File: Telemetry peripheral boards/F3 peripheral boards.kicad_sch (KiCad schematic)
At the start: 39 parts, among them J1 ATS668LSM, J2 Conn_01x04_MountingPin, J3 Potentiometer, J4 Strain Gauge, U1 LM2907M/NOPB, U2 INA125U, U3 MCP2515-I/SO, U4 ISO1050DUB, U5 ATTINY1616-MNR, U6 LM7805_TO220, U7 LD1117V33C

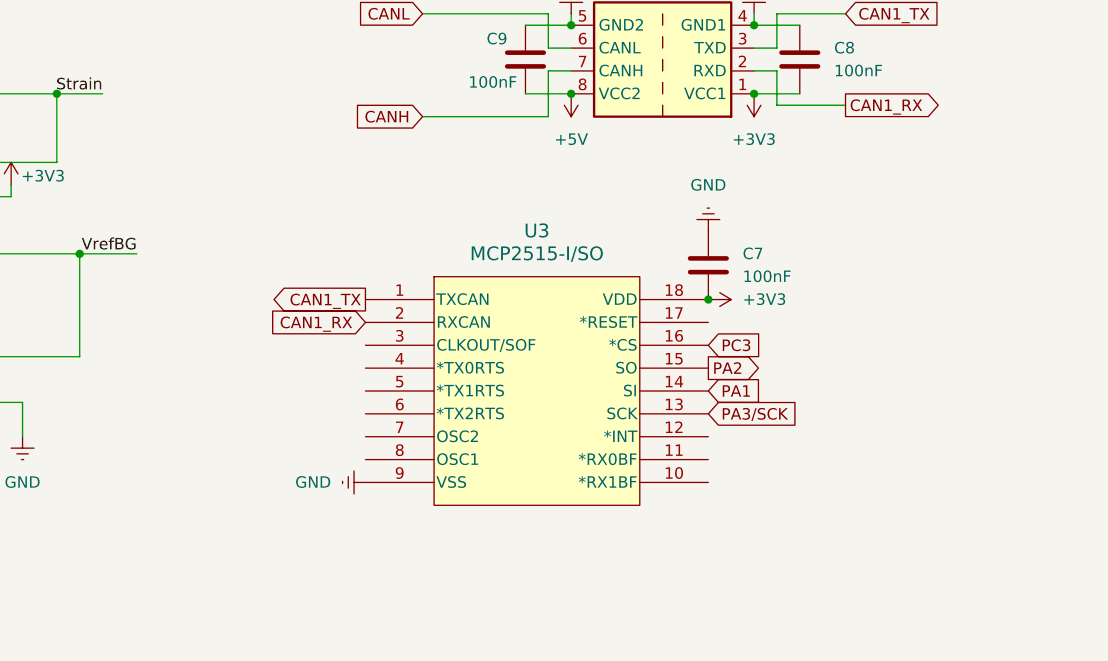
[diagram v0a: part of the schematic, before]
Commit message: updated can controller
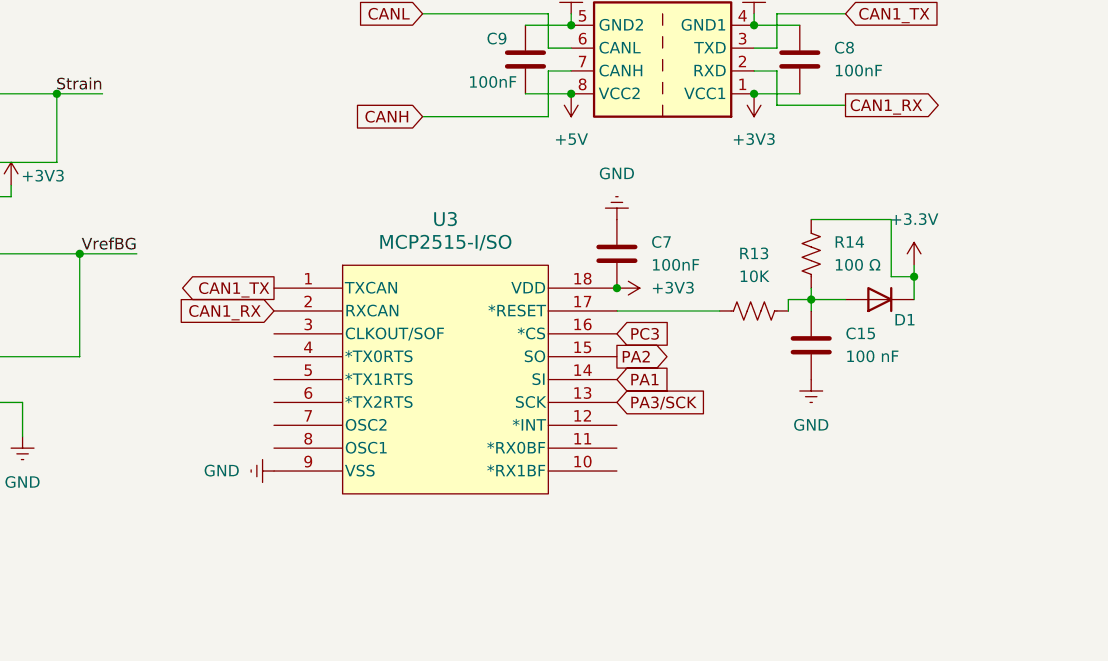
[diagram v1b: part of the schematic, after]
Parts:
- added C15: 100 nF, Capacitor_SMD:C_0805_2012Metric_Pad1.18x1.45mm_HandSolder, symbol Device:C
- added D1: D, Diode_SMD:D_0805_2012Metric, symbol Device:D
- added R13: 10K, Resistor_SMD:R_0805_2012Metric_Pad1.20x1.40mm_HandSolder, symbol Device:R_US
- added R14: 100 Ω, Resistor_SMD:R_0805_2012Metric_Pad1.20x1.40mm_HandSolder, symbol Device:R_US
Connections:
- net GND: now also C15.2
- net at U3.17 (*RESET): now also R13.1
- new net: C15.1, D1.2 (A), R13.2, R14.2
- new net +3.3V: D1.1 (K), R14.1
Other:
- moved on the sheet: C7, U3

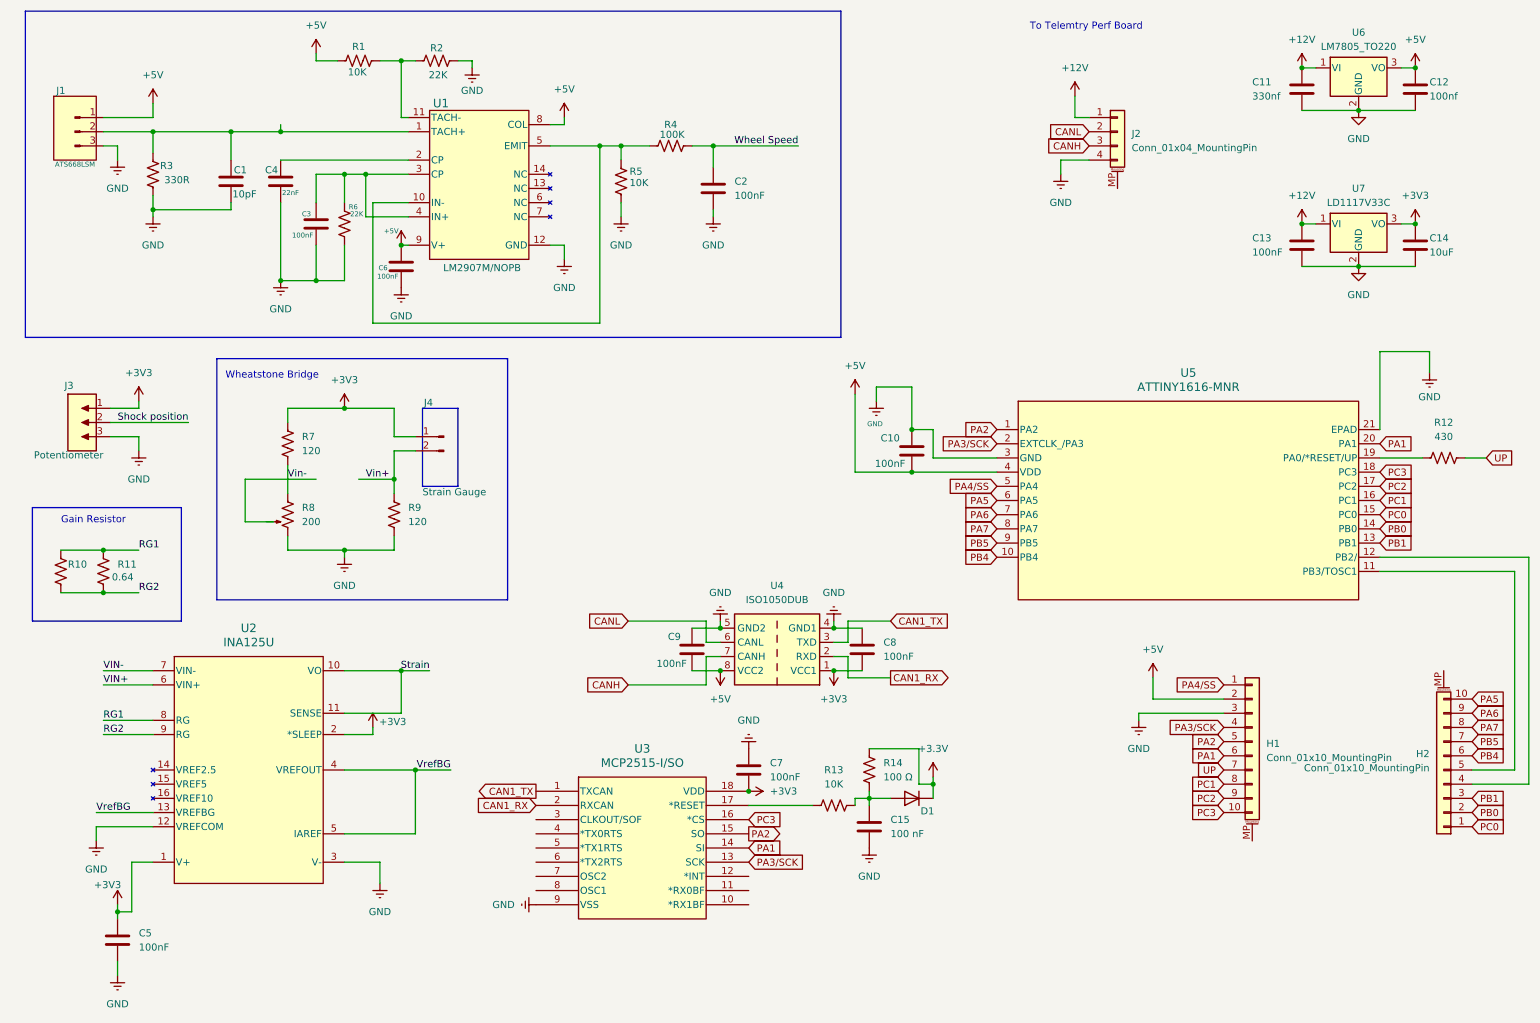
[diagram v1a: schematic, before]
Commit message: PCB for peripheral boards
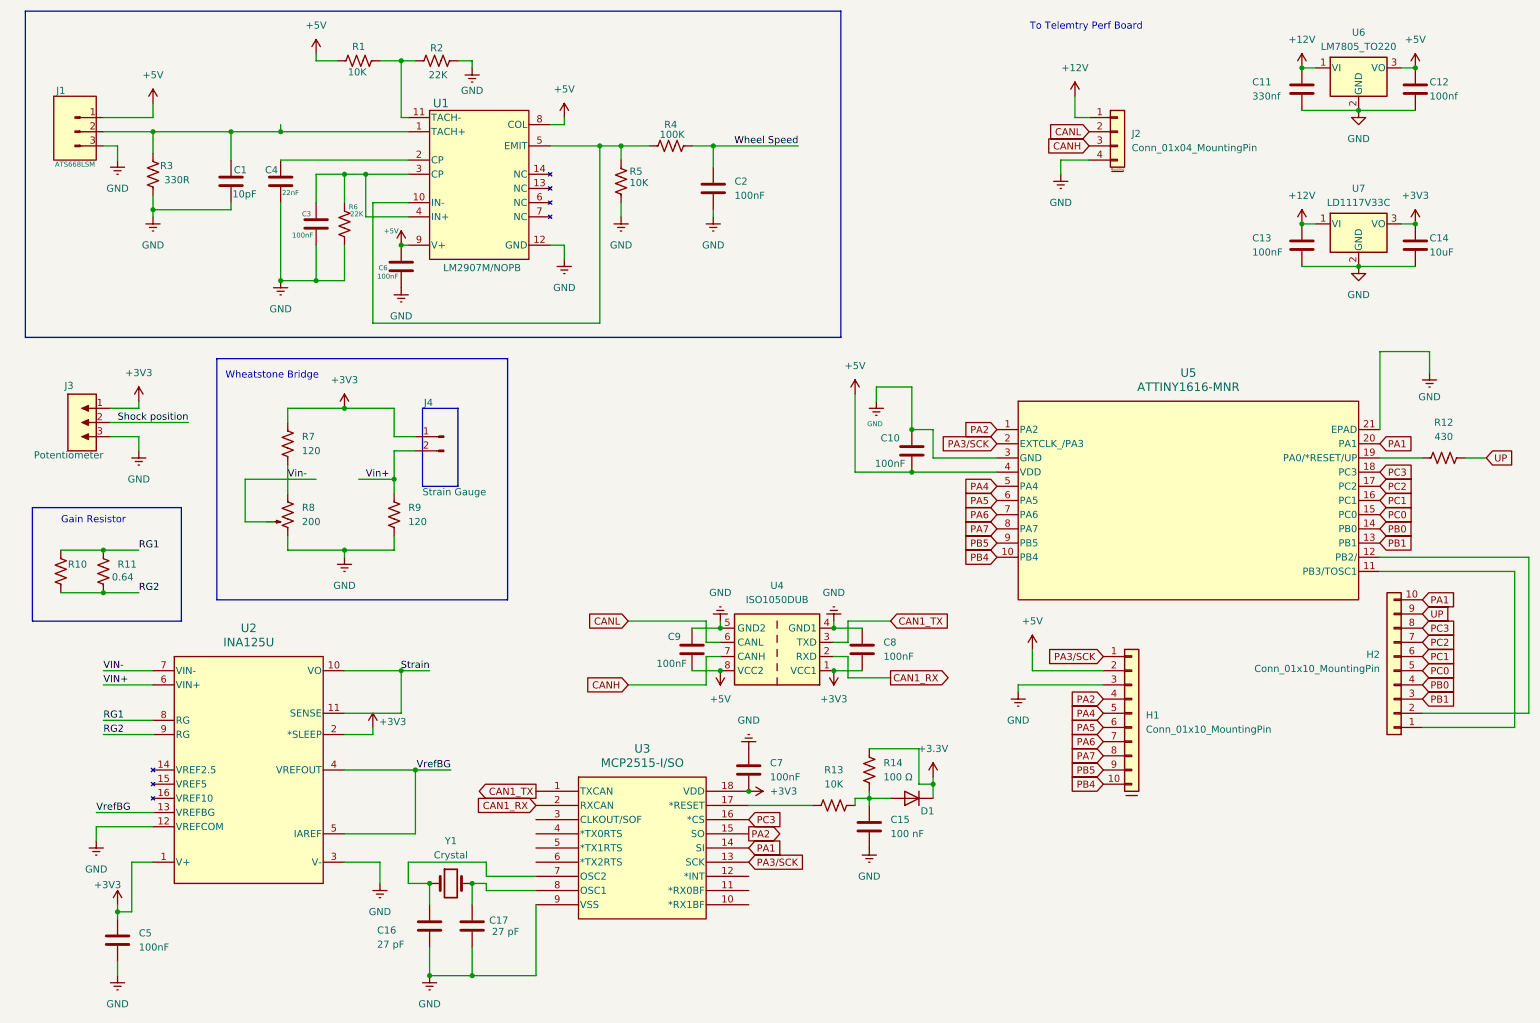
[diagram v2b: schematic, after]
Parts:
- added C16, C17: 27 pF, Capacitor_SMD:C_0805_2012Metric_Pad1.18x1.45mm_HandSolder, symbol Device:C
- added Y1: Crystal, Crystal:Crystal_SMD_5032-2Pin_5.0x3.2mm_HandSoldering, symbol Device:Crystal
- H1: footprint (none) -> Connector_PinHeader_1.00mm:PinHeader_1x10_P1.00mm_Vertical
- J1: footprint (none) -> Connector_PinHeader_2.00mm:PinHeader_1x03_P2.00mm_Vertical
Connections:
- net GND: now also C16.2, C17.2
- net PA1: now also H2.10 (Pin_10); no longer H1.6 (Pin_6)
- net PA2: now also H1.4 (Pin_4); no longer H1.5 (Pin_5)
- net PA3/SCK: now also H1.1 (Pin_1); no longer H1.4 (Pin_4)
- net PA5: now also H1.6 (Pin_6); no longer H2.10 (Pin_10)
- net PA6: now also H1.7 (Pin_7); no longer H2.9 (Pin_9)
- net PA7: now also H1.8 (Pin_8); no longer H2.8 (Pin_8)
- net PB0: now also H2.4 (Pin_4); no longer H2.2 (Pin_2)
- net PB4: now also H1.10 (Pin_10); no longer H2.6 (Pin_6)
- net PB5: now also H1.9 (Pin_9); no longer H2.7 (Pin_7)
- net PC0: now also H2.5 (Pin_5); no longer H2.1 (Pin_1)
- net PC1: now also H2.6 (Pin_6); no longer H1.8 (Pin_8)
- net PC2: now also H2.7 (Pin_7); no longer H1.9 (Pin_9)
- net PC3: now also H2.8 (Pin_8); no longer H1.10 (Pin_10)
- net UP: now also H2.9 (Pin_9); no longer H1.7 (Pin_7)
- net at U5.11 (PB3/TOSC1): now also H2.1 (Pin_1); no longer H2.5 (Pin_5)
- net at U5.12 (PB2/): now also H2.2 (Pin_2); no longer H2.4 (Pin_4)
- net at U3.7 (OSC2): now also C16.1, Y1.1
- net at U3.8 (OSC1): now also C17.1, Y1.2
- net PA4/SS renamed PA4
- net PA4: now also H1.5 (Pin_5); no longer H1.1 (Pin_1)

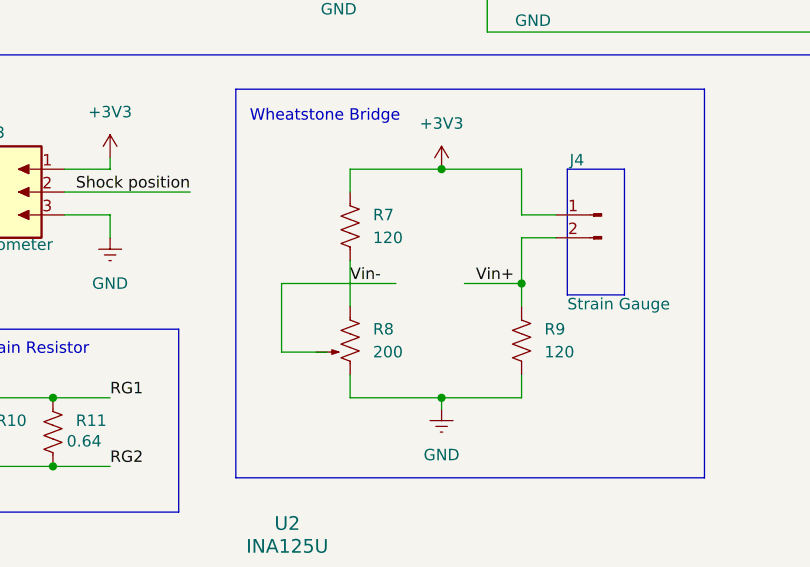
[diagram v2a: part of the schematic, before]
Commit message: Peripheral boards
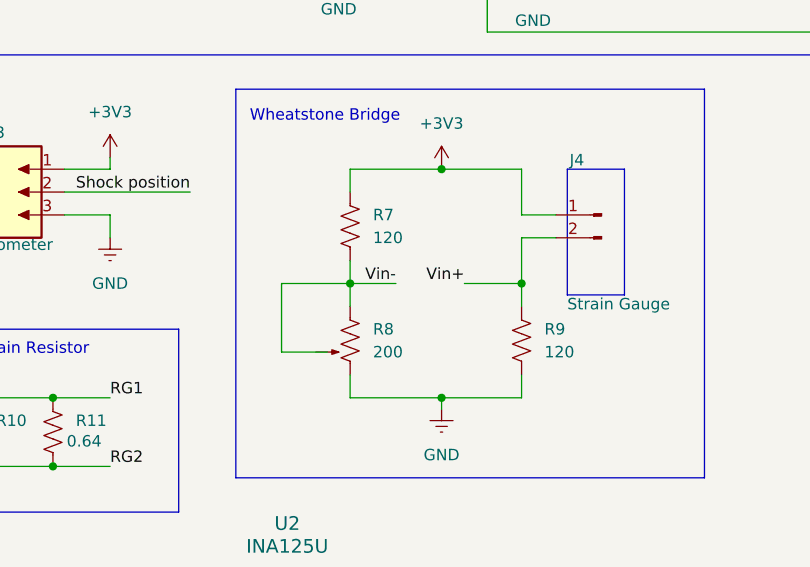
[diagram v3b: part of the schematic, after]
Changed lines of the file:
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@@
+	)
+	(junction
+		(at 60.96 97.79)
+		(diameter 0)
+		(color 0 0 0 0)
 	)
 	(junction
@@
 	(wire
 		(pts
-			(xy 60.96 95.25) (xy 60.96 100.33)
+			(xy 60.96 95.25) (xy 60.96 97.79)
 		)
 		(stroke
@@
 	(wire
 		(pts
+			(xy 60.96 97.79) (xy 53.34 97.79)
+		)
+		(stroke
+			(width 0)
+			(type default)
+		)
+	)
+	(wire
+		(pts
 			(xy 158.75 132.08) (xy 163.83 132.08)
 		)
@@
 	(wire
 		(pts
+			(xy 73.66 97.79) (xy 80.01 97.79)
+		)
+		(stroke
+			(width 0)
+			(type default)
+		)
+	)
+	(wire
+		(pts
 			(xy 172.72 81.28) (xy 166.37 81.28)
 		)
@@
 	(wire
 		(pts
+			(xy 60.96 97.79) (xy 60.96 100.33)
+		)
+		(stroke
+			(width 0)
+			(type default)
+		)
+	)
+	(wire
+		(pts
 			(xy 30.48 38.1) (xy 30.48 40.64)
 		)
@@
 	(wire
 		(pts
-			(xy 66.04 97.79) (xy 53.34 97.79)
-		)
-		(stroke
-			(width 0)
-			(type default)
-		)
-	)
-	(wire
-		(pts
 			(xy 158.75 129.54) (xy 161.29 129.54)
 		)
@@
 	(wire
 		(pts
+			(xy 66.04 97.79) (xy 60.96 97.79)
+		)
+		(stroke
+			(width 0)
+			(type default)
+		)
+	)
+	(wire
+		(pts
 			(xy 176.53 93.98) (xy 176.53 88.9)
 		)
@@
 		(pts
 			(xy 80.01 107.95) (xy 80.01 110.49)
-		)
-		(stroke
-			(width 0)
-			(type default)
-		)
-	)
-	(wire
-		(pts
-			(xy 73.66 97.79) (xy 80.01 97.79)
 		)
 		(stroke
@@
 	)
 	(label "Vin-"
-		(at 60.96 97.79 0)
+		(at 66.04 97.79 180)
 		(fields_autoplaced yes)
 		(effects
@@
 				(size 1.27 1.27)
 			)
-			(justify left bottom)
+			(justify right bottom)
 		)
 	)
@@
 	)
 	(label "Vin+"
-		(at 74.93 97.79 0)
+		(at 73.66 97.79 180)
 		(fields_autoplaced yes)
 		(effects
@@
 				(size 1.27 1.27)
 			)
-			(justify left bottom)
-		)
-	)
+			(justify right bottom)
+		)
+	)

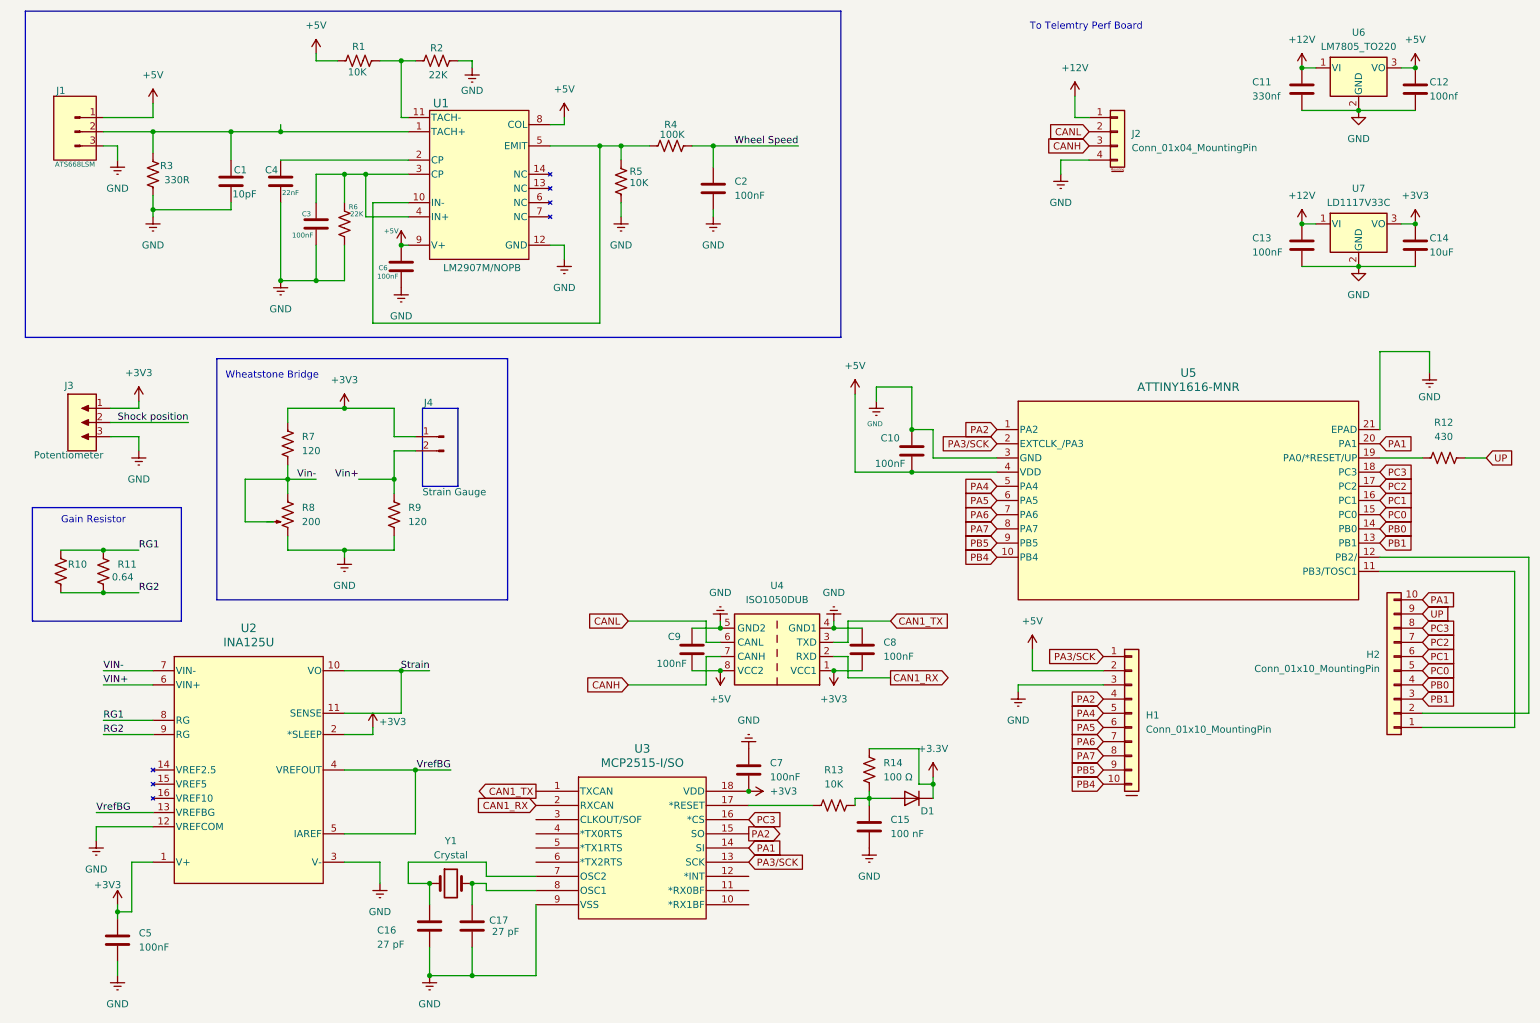
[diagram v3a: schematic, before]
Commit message: Update With Tire Temp Sensor
Update With Tire Temp Sensor
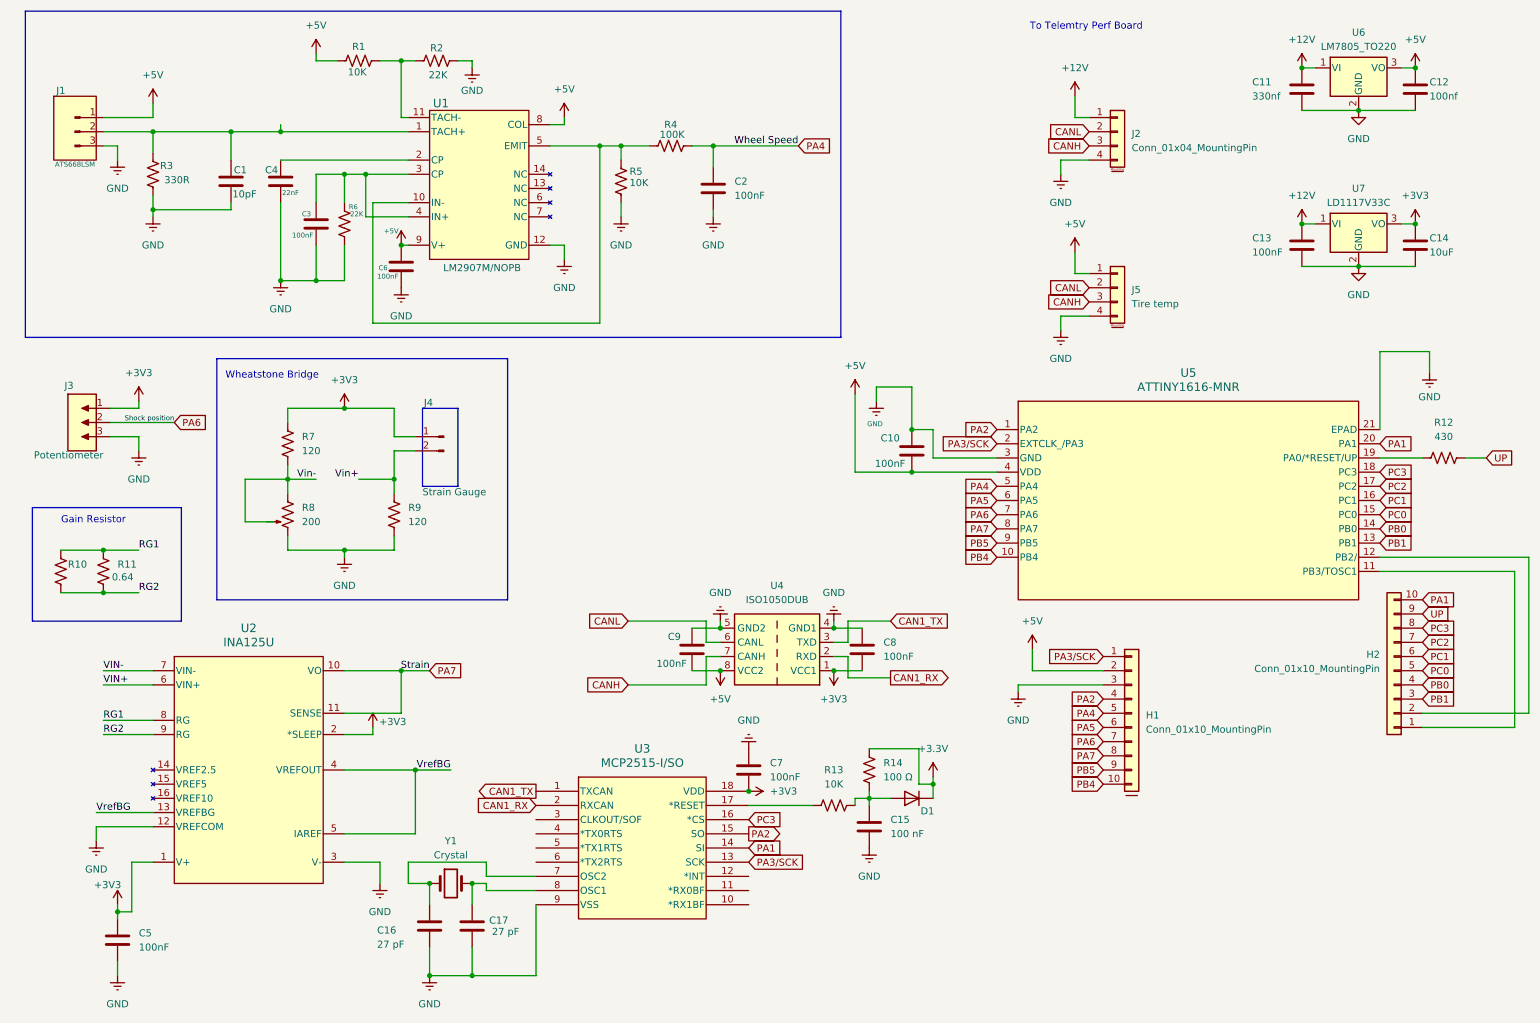
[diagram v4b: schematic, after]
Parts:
- added J5: Tire temp, Connector_PinHeader_1.00mm:PinHeader_1x04_P1.00mm_Vertical, symbol Connector_Generic_MountingPin:Conn_01x04_MountingPin
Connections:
- net Shock position is gone; now on net PA6: J3.2
- net Strain is gone; now on net PA7: U2.10 (VO), U2.11 (SENSE)
- net Wheel Speed is gone; now on net PA4: C2.1, R4.2
- net +5V: now also J5.1 (Pin_1)
- net CANH: now also J5.3 (Pin_3)
- net CANL: now also J5.2 (Pin_2)
- net GND: now also J5.4 (Pin_4)
